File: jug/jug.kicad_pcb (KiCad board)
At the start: 2 copper layers, 153.5 x 107.4 mm, 64 parts, among them J1 USB_A, U1 RP2040_Zero

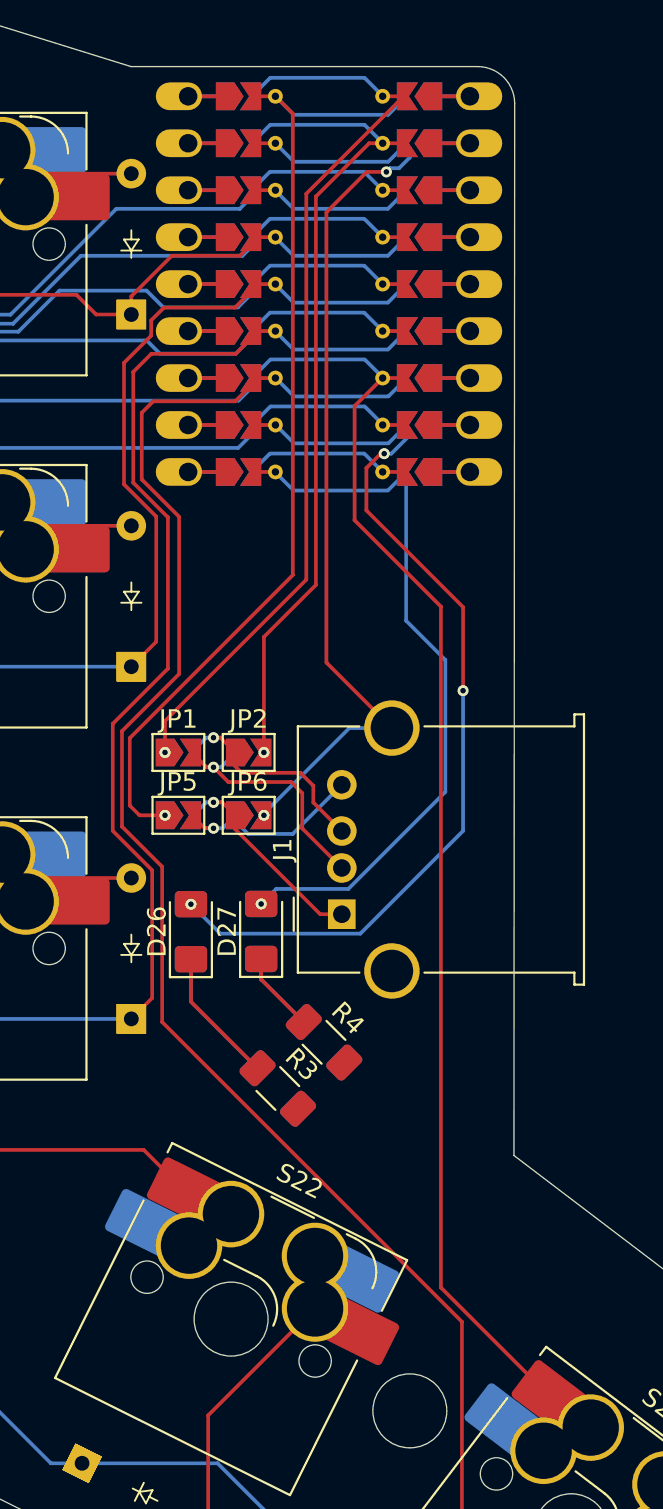
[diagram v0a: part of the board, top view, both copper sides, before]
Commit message: finished pcb
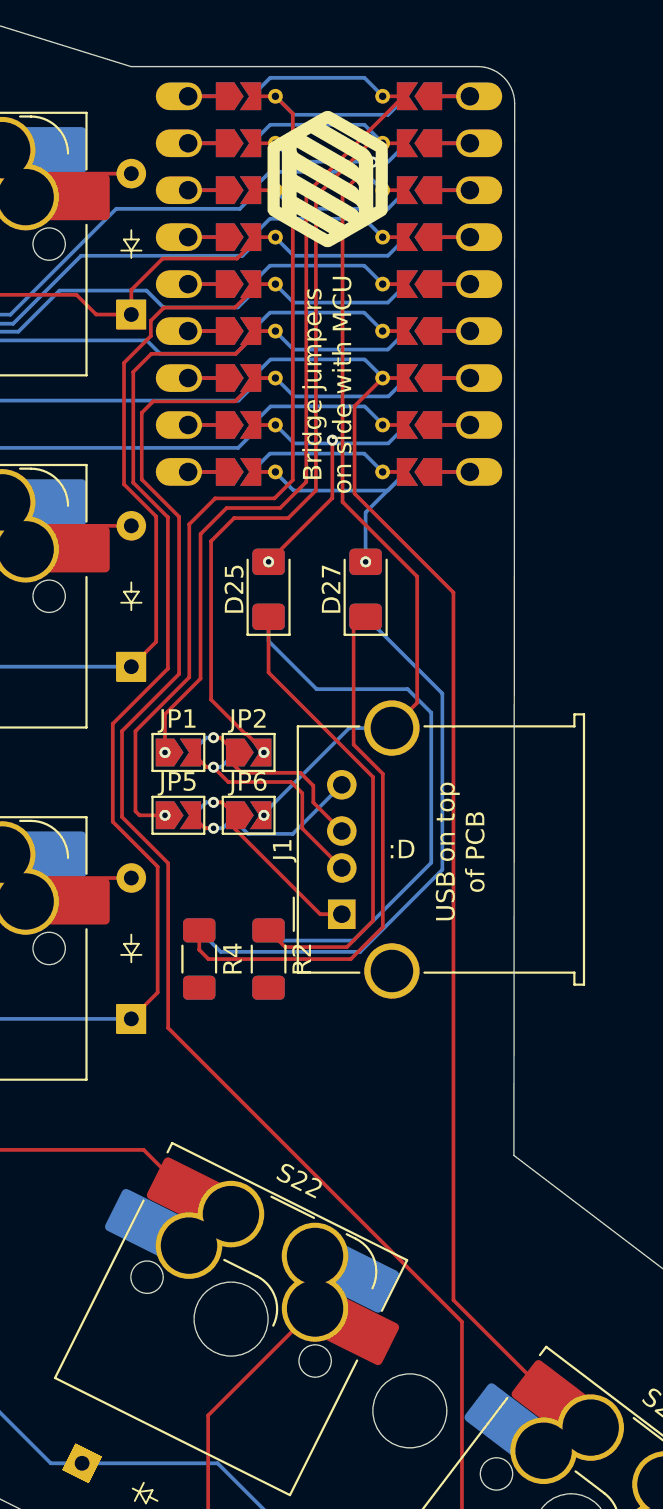
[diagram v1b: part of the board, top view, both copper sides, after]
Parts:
- added G***: LOGO, LOGO, F.Cu at (189.1, 74.0)
- added G***: LOGO, LOGO, B.Cu at (189.1, 74.0)
- D25, R2: moved to F.Cu
- D26, R3: moved to B.Cu
- moved D26 20.8 mm to (191.1, 96.2)
- moved D27 19.3 mm to (191.1, 96.2)
- moved D24 19.0 mm to (185.9, 96.2)
- moved D25 18.5 mm to (185.9, 96.2)
- moved R3 8.19 mm to (182.1, 116.2), turned to -90 degrees
- moved R4 8.11 mm to (182.1, 116.2), turned to -90 degrees
- moved R1 7.02 mm to (185.9, 116.2), turned to -90 degrees
- moved R2 5.41 mm to (185.9, 116.2), turned to -90 degrees
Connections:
- D25 pad 2: LED1 -> LED0
- D26 pad 2: LED0 -> LED1
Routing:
- net LED0: track 42.8 -> 8.01 mm, vias 3 -> 2
- net Net-(D27-K): track 4.37 -> 29.6 mm
- net LED1: track 30.4 -> 5.77 mm
- net Net-(D26-K): track 7.39 -> 30.9 mm
- net Net-(D24-K): track 7.39 -> 30.6 mm
- net Net-(D25-K): track 4.37 -> 25.4 mm
- net INTERCONNECT_B: track 35.7 -> 39.8 mm
- net GND: track 44.6 -> 42.5 mm
- net INTERCONNECT_A: track 40.8 -> 42.5 mm
- net +5V: track 44.2 -> 45.8 mm
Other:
- board text added: ":D"
- board text added: "Bridge jumpers on side with MCU"
- board text added: "USB on top of PCB"
